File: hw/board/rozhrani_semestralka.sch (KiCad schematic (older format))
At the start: 56 parts, among them P1 DISPLAY_CONN, P2 DISPLAY_VCC_CON, P3 USB_B, U1 MCP2210, U2 MIC5504-3.3, U3 Joystick, U4 LM239, U5 CD4532, U6 NPIC6c596, U7 NE555, U8 BS800N, U9 BS800N

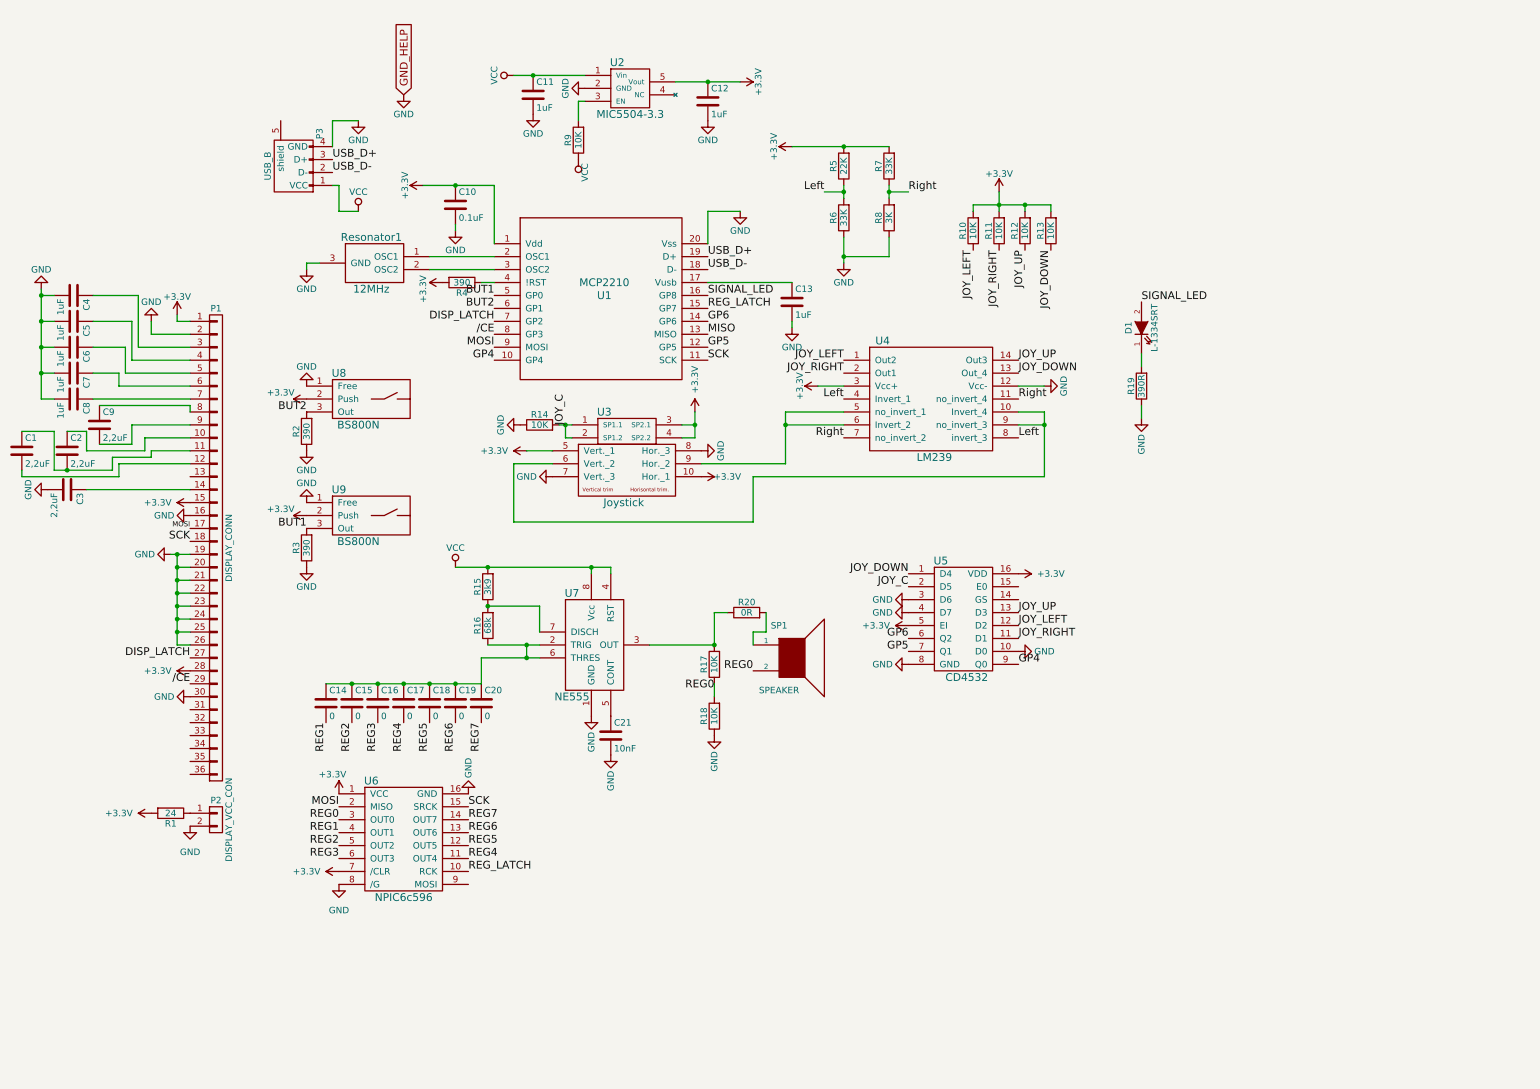
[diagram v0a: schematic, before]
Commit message: Sorting schematic parts
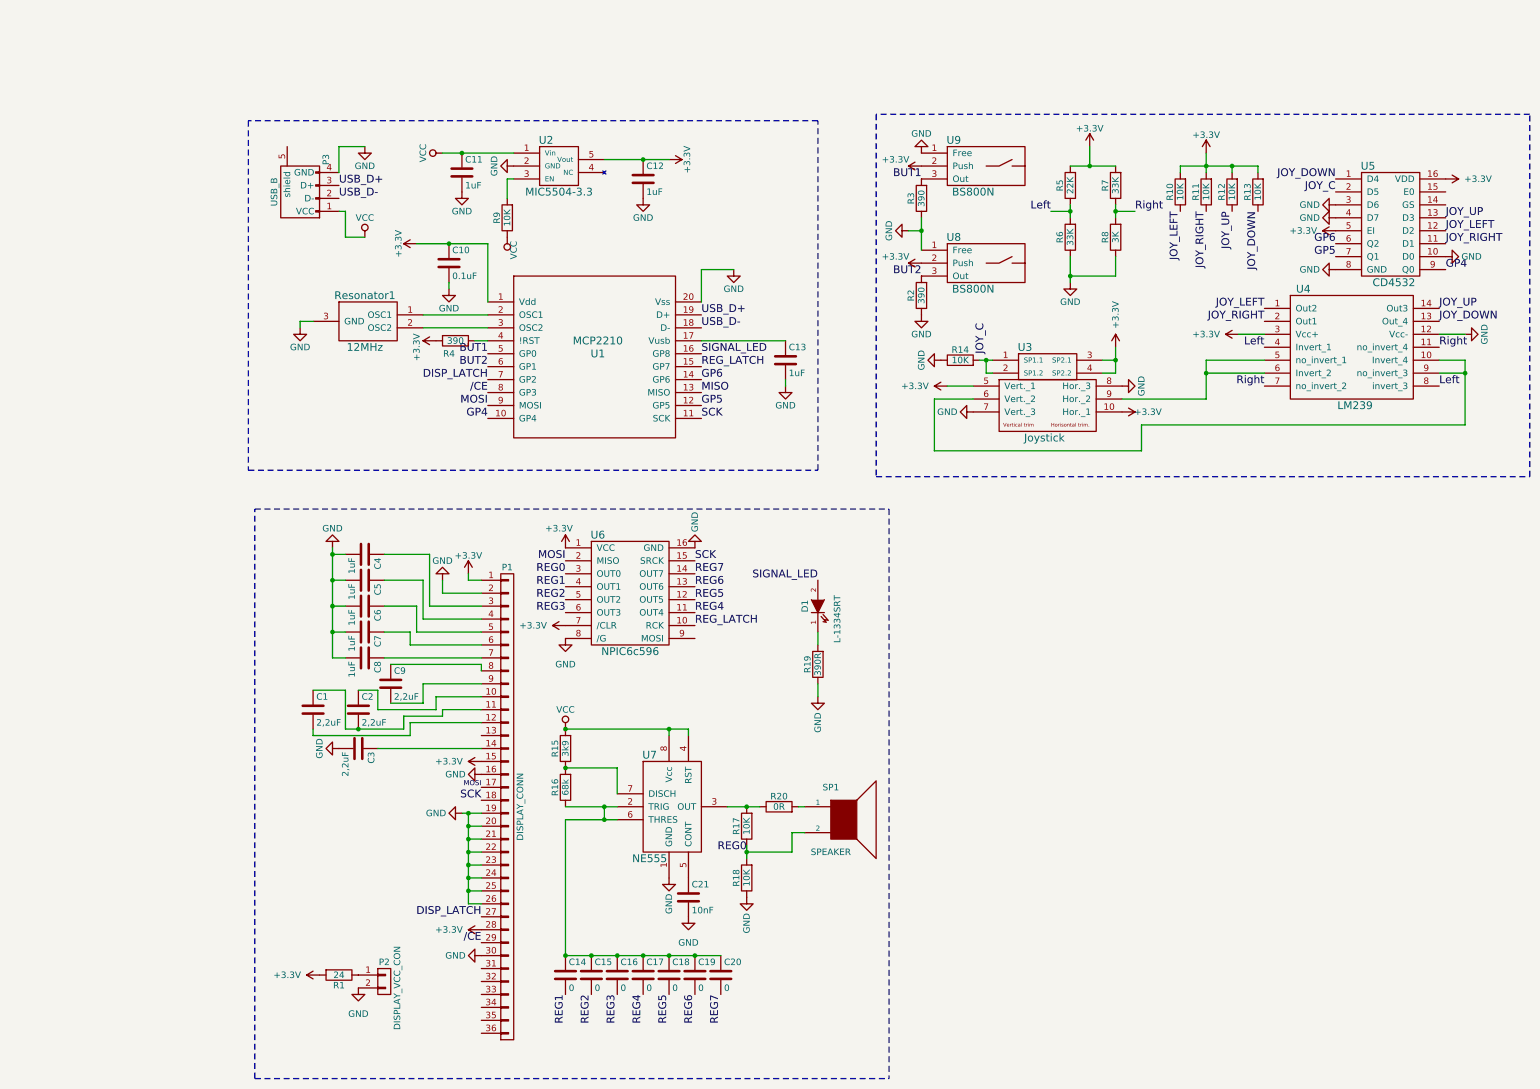
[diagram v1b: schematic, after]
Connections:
- net JOY_C: no longer R14.2, U3.1 (SP1.1), U3.2 (SP1.2)
- new net: R14.2, U3.1 (SP1.1), U3.2 (SP1.2)
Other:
- moved on the sheet: C1, C10, C11, C12, C13, C14, C15, C16, C17, C18, C19, C2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
